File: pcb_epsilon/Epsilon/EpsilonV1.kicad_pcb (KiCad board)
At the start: 2 copper layers, 29 x 11.5 mm, 18 parts, among them J1 SG1m, J2 SG2p, J3 SG1p, J4 SG2m, Q1 AO3401A, U1 ADA4940-1ARZ-R7, U2 DS28E07P+T

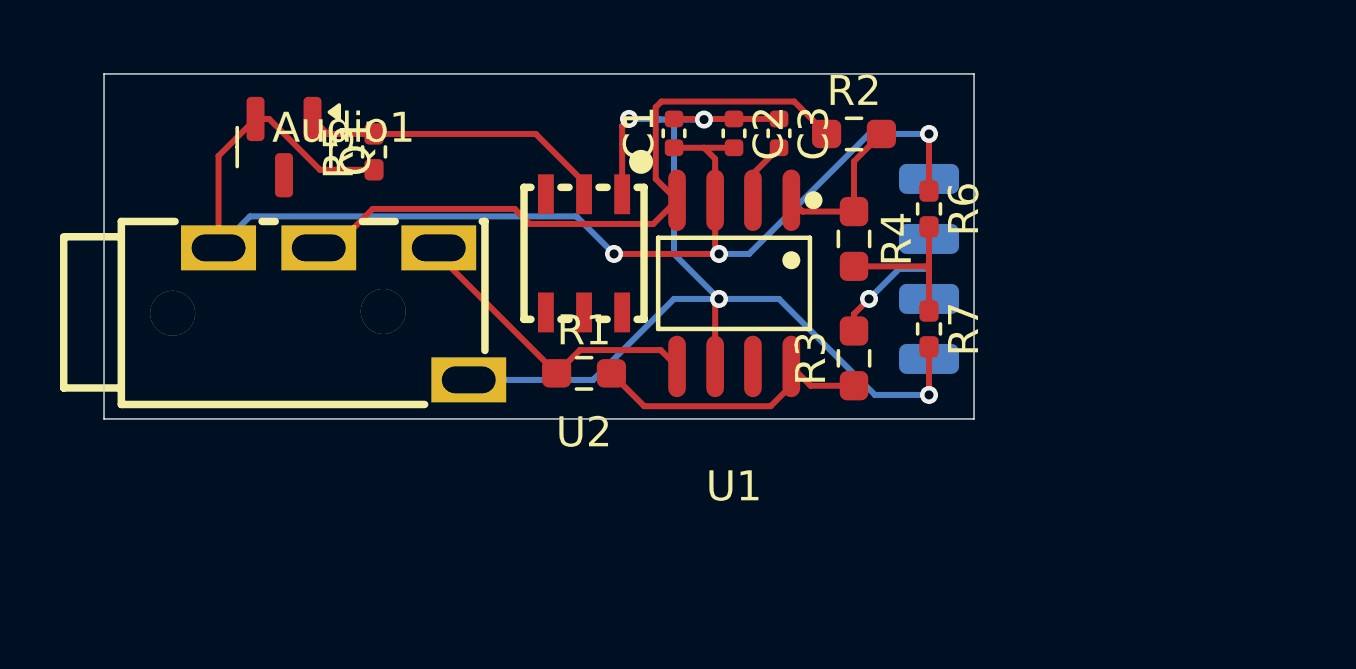
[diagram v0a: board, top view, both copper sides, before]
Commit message: Yolo
Nothing could go wrong
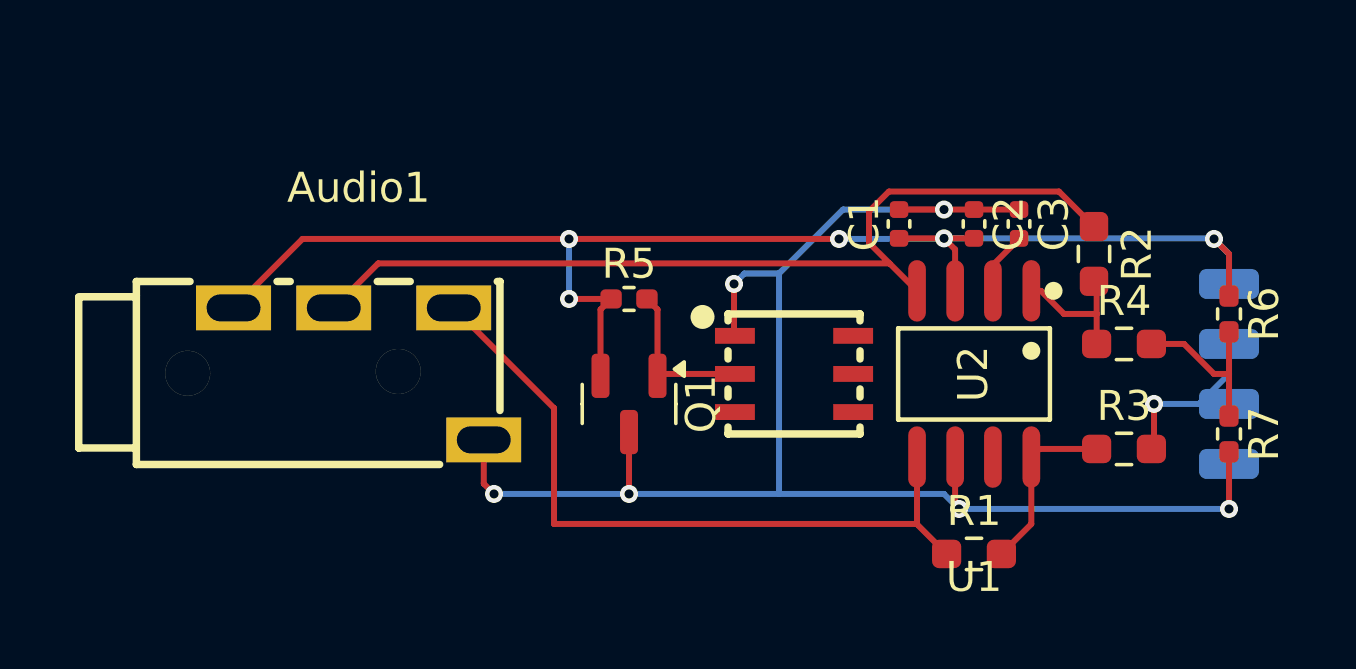
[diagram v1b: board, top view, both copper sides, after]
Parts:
- moved Q1 14.3 mm to (159.0, 131.0)
- moved R1 14.3 mm to (170.5, 136.0)
- moved J1 10.6 mm to (179.0, 129.0)
- moved J2 10.6 mm to (179.0, 131.0)
- moved J3 10.6 mm to (179.0, 127.0)
- moved J4 10.6 mm to (179.0, 133.0)
- moved R6 10.6 mm to (179.0, 128.0)
- moved R7 10.6 mm to (179.0, 132.0)
- moved R5 9.81 mm to (159.0, 127.5), turned to 0 degrees
- moved R4 9.66 mm to (175.5, 129.0), turned to 0 degrees
- moved R3 9.49 mm to (175.5, 132.5), turned to 0 degrees
- moved R2 8.94 mm to (174.5, 126.0), turned to -90 degrees
- moved C2 8.55 mm to (170.5, 125.0)
- moved C3 8.55 mm to (172.0, 125.0)
- moved U1 8.55 mm to (170.5, 130.0)
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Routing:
- net GND: track 38.1 -> 55.0 mm, vias 4 -> 6
- net Net-(U1-–OUT): track 10.4 -> 24.3 mm
- net Net-(U1-+OUT): track 22.6 -> 30.7 mm
- net Net-(Q1-G): track 10.3 -> 5.31 mm
- net Net-(U1-+IN): track 9.73 -> 5.93 mm
- net 3V3A_SW: track 44.9 -> 48.0 mm, vias 3 -> 5
- net Net-(J1-Pin_1): track 5.69 -> 6.45 mm
- net Net-(U1-–IN): track 5.21 -> 4.62 mm
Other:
- board outline removed
